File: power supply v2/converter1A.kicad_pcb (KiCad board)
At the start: 2 copper layers, 38.3 x 37.5 mm, 45 parts, among them IC2 LM25145RGYR, IC3 LMR50410YQDBVRQ1, J1 1933189, J3 1933189, J4 Conn_01x04_Pin, Q1 CSD17577Q3A, Q2 CSD17577Q3A

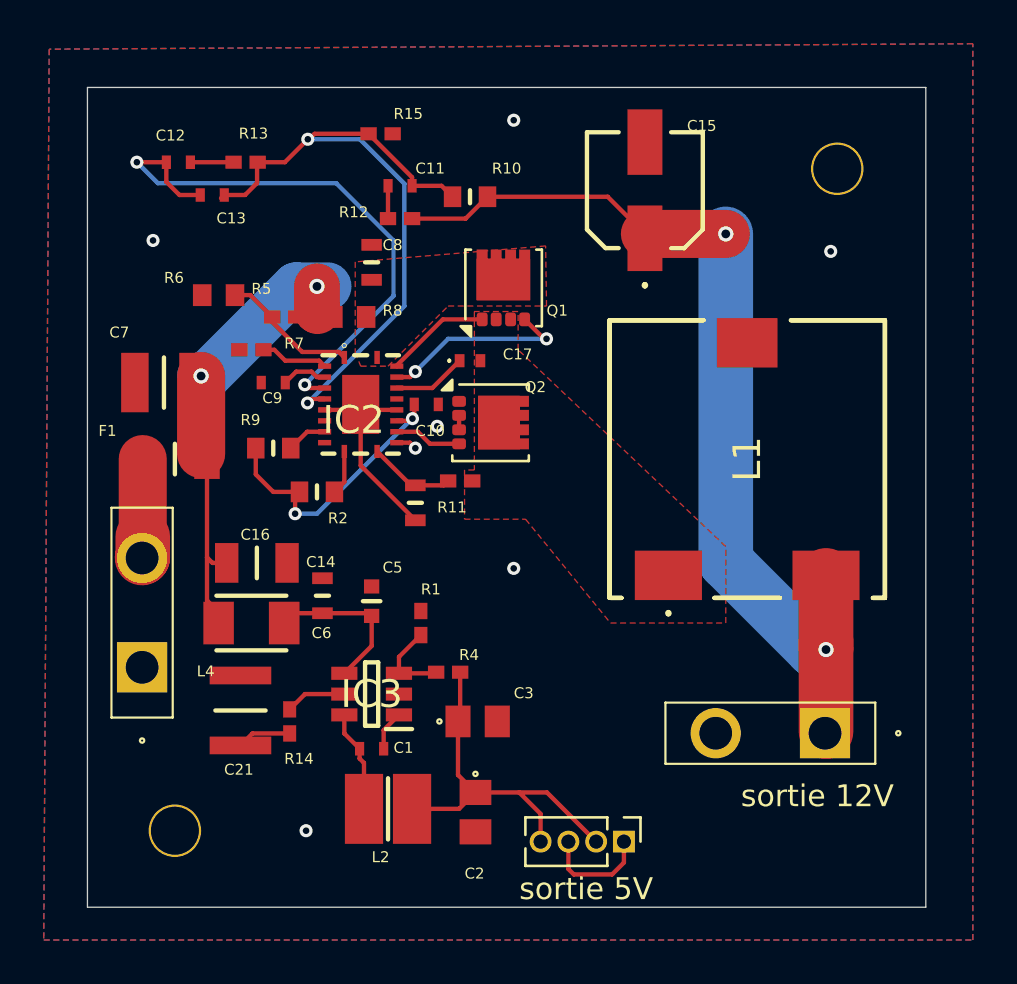
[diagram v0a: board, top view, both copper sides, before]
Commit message: last version of pcb and gerber files
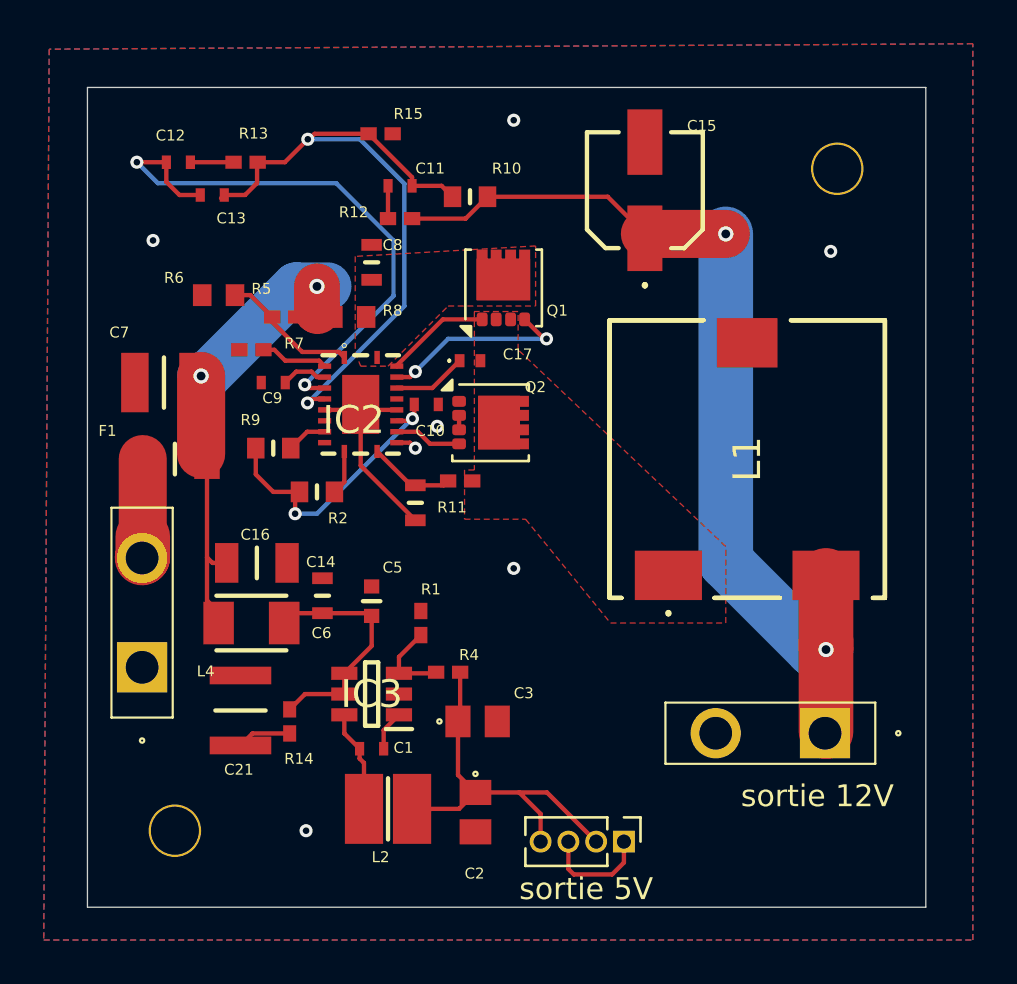
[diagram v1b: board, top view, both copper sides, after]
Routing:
- net Net-(IC3-EN): track 10.2 -> 11.1 mm
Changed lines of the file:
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@@
 			(plot_on_all_layers_selection 0x00000000_00000000_00000000_00000000)
 			(disableapertmacros no)
-			(usegerberextensions no)
+			(usegerberextensions yes)
 			(usegerberattributes yes)
 			(usegerberadvancedattributes yes)
-			(creategerberjobfile yes)
+			(creategerberjobfile no)
 			(dashed_line_dash_ratio 12.000000)
 			(dashed_line_gap_ratio 3.000000)
@@
 			(sketchdnponfab yes)
 			(crossoutdnponfab yes)
-			(subtractmaskfromsilk no)
+			(subtractmaskfromsilk yes)
 			(outputformat 1)
 			(mirror no)
-			(drillshape 1)
+			(drillshape 0)
 			(scaleselection 1)
-			(outputdirectory "")
+			(outputdirectory "gerber files/")
 		)
 	)
@@
 	)
 	(segment
+		(start 175.75 100.8)
+		(end 175.75 101.75)
+		(width 0.2)
+		(layer "F.Cu")
+		(net 1)
+	)
+	(segment
 		(start 176.875 98.05)
 		(end 177 98.175)
@@
 		(polygon
 			(pts
-				(xy 181.7 84.25) (xy 181.7 84.25) (xy 181.7 91.5) (xy 181.25 91.5) (xy 181.25 93.75) (xy 184.040911 93.75)
-				(xy 187.927275 98.5) (xy 193.2 98.5) (xy 193.2 95) (xy 183.7 86) (xy 183.7 84.25)
+				(xy 181.7 84.25) (xy 181.7 91.5) (xy 181.25 91.5) (xy 181.25 93.75) (xy 184.040911 93.75) (xy 187.927275 98.5)
+				(xy 193.2 98.5) (xy 193.2 95) (xy 183.7 86) (xy 183.7 84.25)
 			)
 		)
@@
 		(polygon
 			(pts
-				(xy 176.25 86.125) (xy 176.5 86.75) (xy 177.75 86.75) (xy 180.5 84) (xy 185 84) (xy 184.959276 81.25)
-				(xy 176.25 81.979072)
+				(xy 176.25 86.125) (xy 176.5 86.75) (xy 177.75 86.75) (xy 180.5 84) (xy 184.5 84) (xy 184.5 81.25)
+				(xy 176.25 81.729072)
 			)
 		)
